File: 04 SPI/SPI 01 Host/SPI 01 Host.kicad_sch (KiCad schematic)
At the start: 20 parts, among them J101 ICSP, J102 USB_A, SW101 SW_DIP_x08, U1 MCP23S17_SO, U101 PIC18F47Q43-I/PT, U103 FT232RL, U2 74LS138

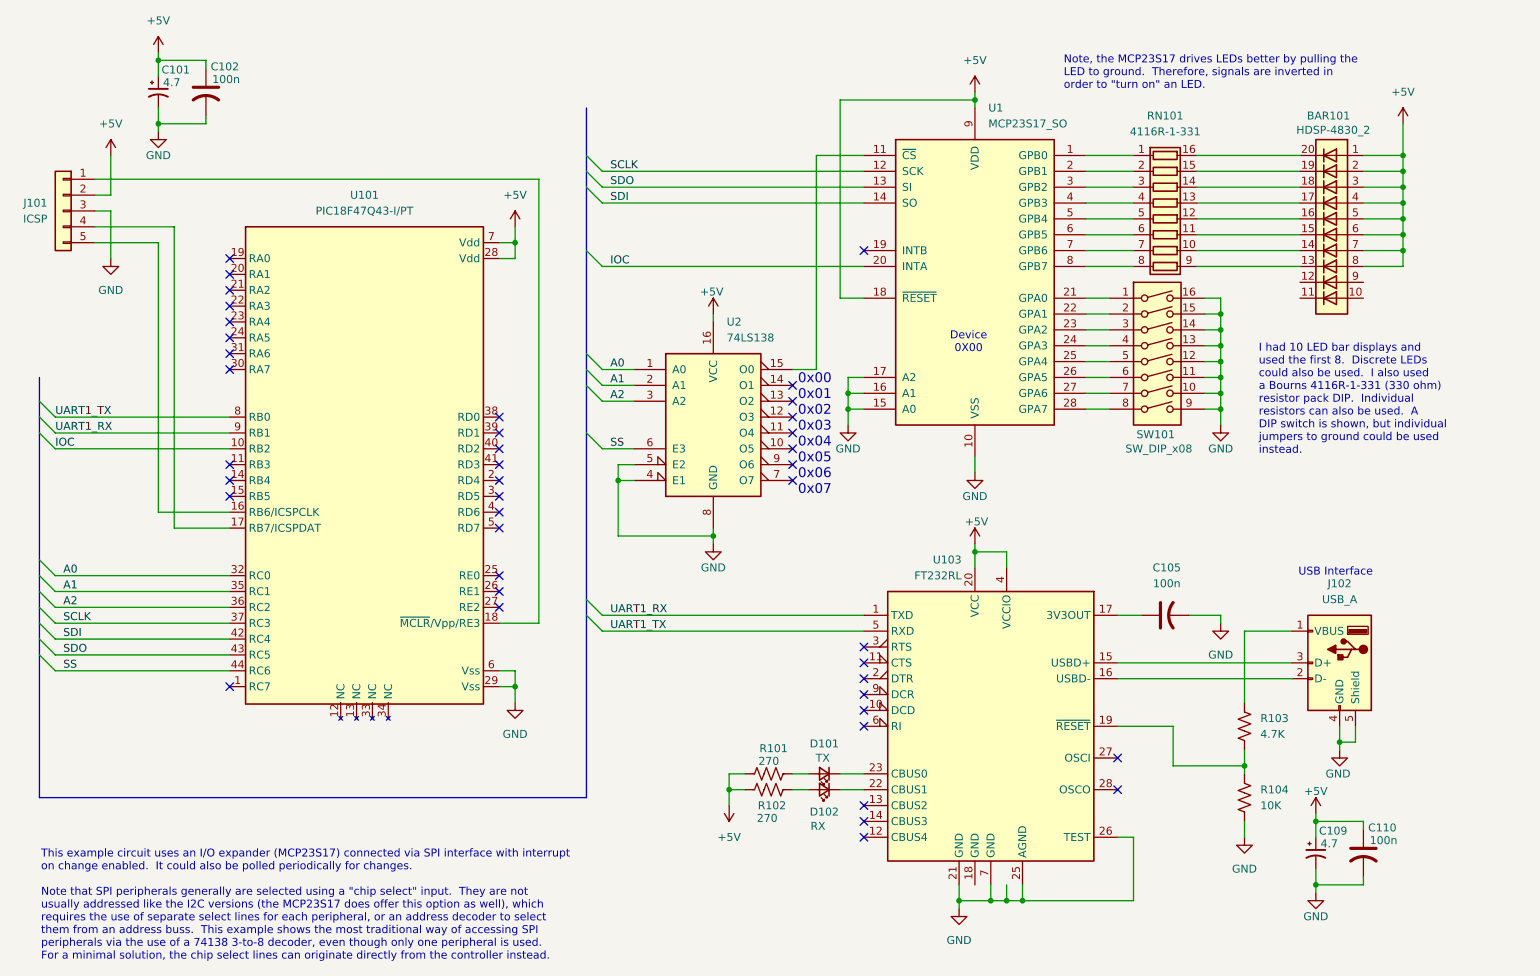
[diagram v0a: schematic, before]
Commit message: spi
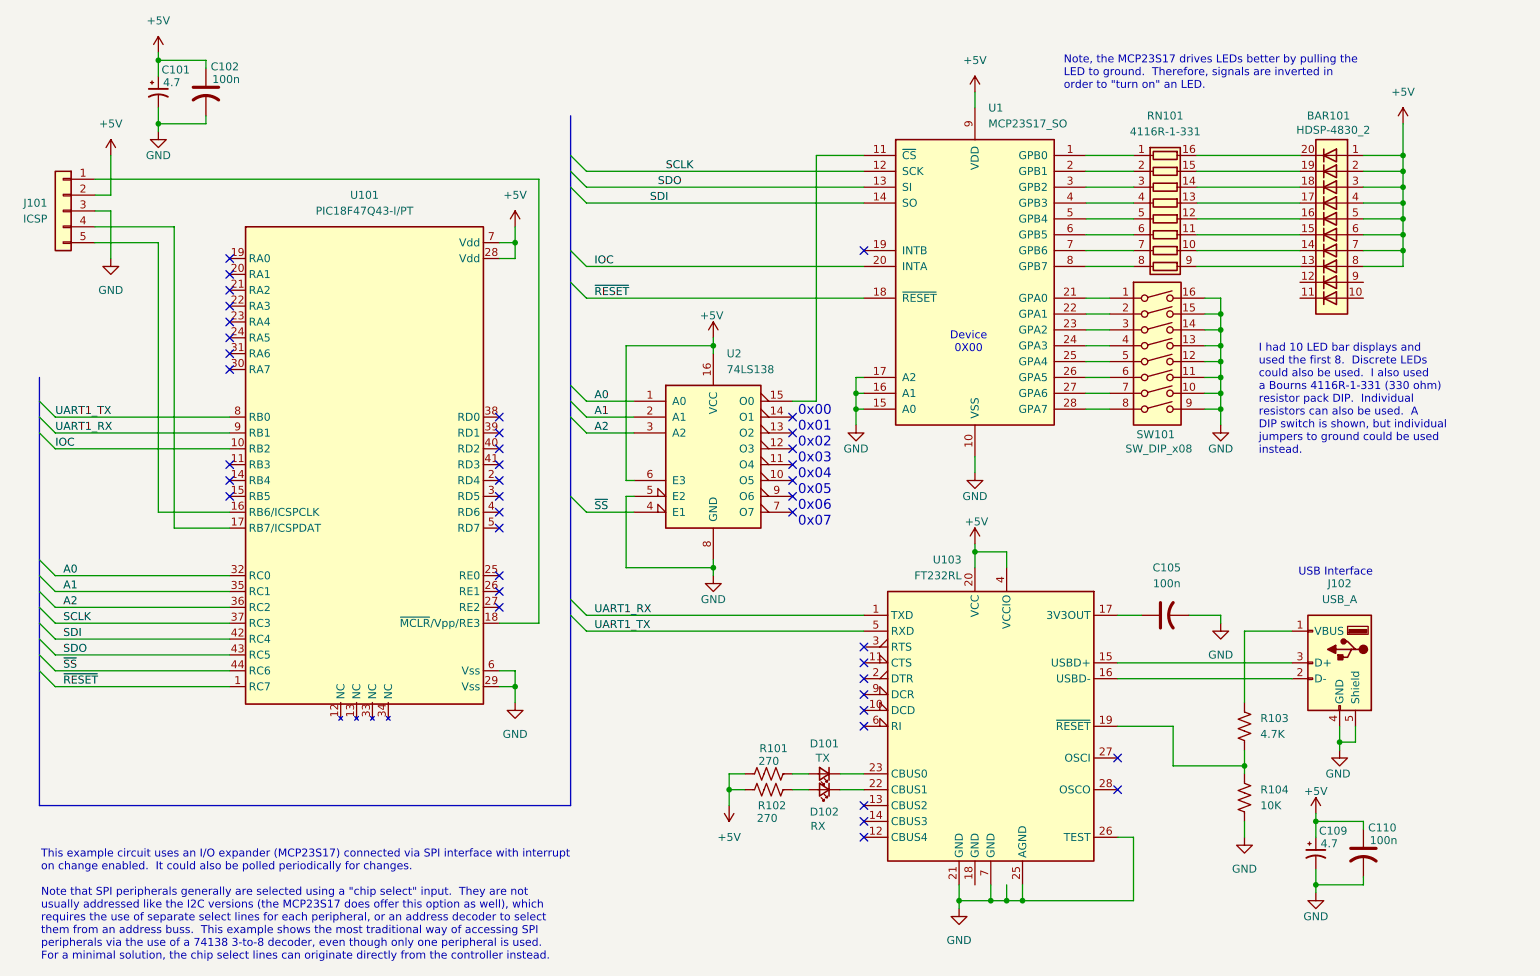
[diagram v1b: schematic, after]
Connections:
- net +5V: now also U2.6 (E3); no longer U1.18 (~{RESET})
- net GND: no longer U2.4 (E1)
- net ~{RESET}: now reaches U101.1 (RC7)
- net ~{RESET}: now also U1.18 (~{RESET})
- net SS renamed ~{SS}
- net ~{SS}: now also U2.4 (E1); no longer U2.6 (E3)
- no-connect marks 42 -> 41
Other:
- moved on the sheet: U2
